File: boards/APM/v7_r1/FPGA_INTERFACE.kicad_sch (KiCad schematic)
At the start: 30 parts, among them J1 DF40C-60DS-0.4V(51), J15 FPGA FFC, J21 FPGA FMC, J3 DF40C-60DS-0.4V(51), J31 Conn_02x04_Odd_Even, SW1 RST

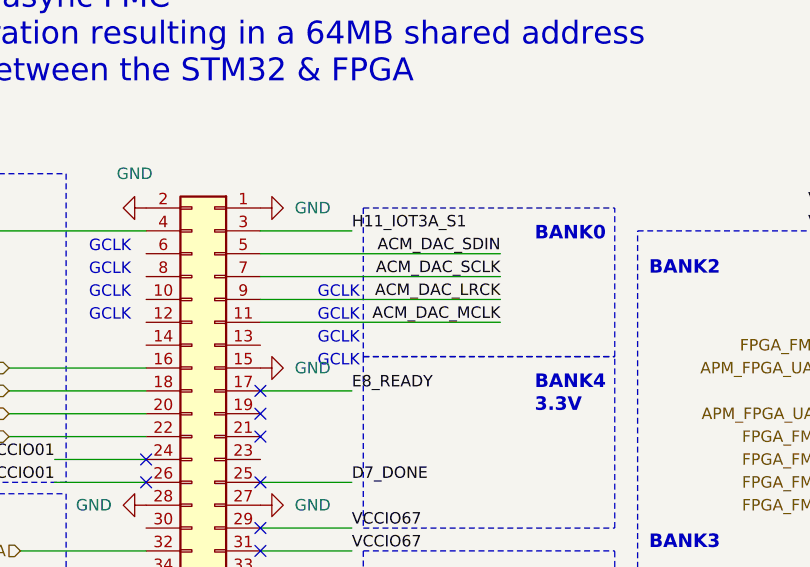
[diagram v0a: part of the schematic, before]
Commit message: floorplanning again
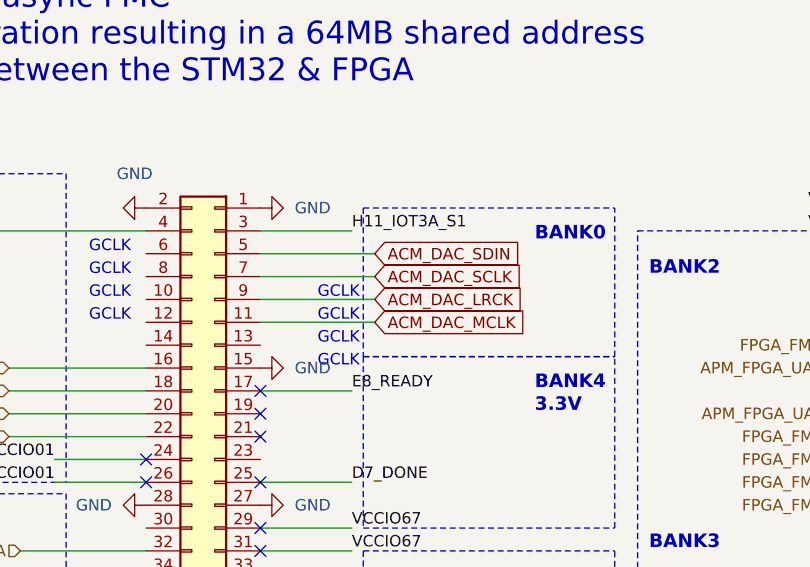
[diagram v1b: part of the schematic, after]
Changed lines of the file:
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@@
 	(wire
 		(pts
-			(xy 95.25 96.52) (xy 68.58 96.52)
+			(xy 81.28 96.52) (xy 68.58 96.52)
 		)
 		(stroke
@@
 	(wire
 		(pts
-			(xy 95.25 99.06) (xy 68.58 99.06)
+			(xy 81.28 99.06) (xy 68.58 99.06)
 		)
 		(stroke
@@
 	(wire
 		(pts
-			(xy 95.25 101.6) (xy 68.58 101.6)
+			(xy 81.28 101.6) (xy 68.58 101.6)
 		)
 		(stroke
@@
 	(wire
 		(pts
-			(xy 95.25 93.98) (xy 68.58 93.98)
+			(xy 81.28 93.98) (xy 68.58 93.98)
 		)
 		(stroke
@@
 		)
 	)
-	(label "ACM_DAC_MCLK"
-		(at 95.25 101.6 180)
-		(effects
-			(font
-				(size 1.27 1.27)
-			)
-			(justify right bottom)
-		)
-	)
 	(label "A3_JTAG_TDI"
 		(at 166.37 121.92 0)
@@
 		)
 	)
-	(label "ACM_DAC_LRCK"
-		(at 95.25 99.06 180)
-		(effects
-			(font
-				(size 1.27 1.27)
-			)
-			(justify right bottom)
-		)
-	)
 	(label "FPGA_3V3"
 		(at 137.16 149.86 180)
@@
 		)
 	)
-	(label "ACM_DAC_SDIN"
-		(at 95.25 93.98 180)
-		(effects
-			(font
-				(size 1.27 1.27)
-			)
-			(justify right bottom)
-		)
-	)
 	(label "FPGA_3V3"
 		(at 95.25 181.61 0)
@@
 		)
 	)
-	(label "ACM_DAC_SCLK"
-		(at 95.25 96.52 180)
-		(effects
-			(font
-				(size 1.27 1.27)
-			)
-			(justify right bottom)
-		)
-	)
 	(label "FPGA_3V3"
 		(at 137.16 147.32 180)
@@
 		)
 	)
+	(global_label "ACM_DAC_SCLK"
+		(shape input)
+		(at 81.28 96.52 0)
+		(fields_autoplaced yes)
+		(effects
+			(font
+				(size 1.27 1.27)
+			)
+			(justify left)
+		)
+		(property "Intersheetrefs" "${INTERSHEET_REFS}"
+			(at 98.4166 96.52 0)
+			(hide yes)
+			(show_name no)
+			(do_not_autoplace no)
+			(effects
+				(font
+					(size 1.27 1.27)
+				)
+				(justify left)
+			)
+		)
+	)
+	(global_label "ACM_DAC_SDIN"
+		(shape input)
+		(at 81.28 93.98 0)
+		(fields_autoplaced yes)
+		(effects
+			(font
+				(size 1.27 1.27)
+			)
+			(justify left)
+		)
+		(property "Intersheetrefs" "${INTERSHEET_REFS}"
+			(at 98.0538 93.98 0)
+			(hide yes)
+			(show_name no)
+			(do_not_autoplace no)
+			(effects
+				(font
+					(size 1.27 1.27)
+				)
+				(justify left)
+			)
+		)
+	)
+	(global_label "ACM_DAC_LRCK"
+		(shape input)
+		(at 81.28 99.06 0)
+		(fields_autoplaced yes)
+		(effects
+			(font
+				(size 1.27 1.27)
+			)
+			(justify left)
+		)
+		(property "Intersheetrefs" "${INTERSHEET_REFS}"
+			(at 98.4771 99.06 0)
+			(hide yes)
+			(show_name no)
+			(do_not_autoplace no)
+			(effects
+				(font
+					(size 1.27 1.27)
+				)
+				(justify left)
+			)
+		)
+	)
+	(global_label "ACM_DAC_MCLK"
+		(shape input)
+		(at 81.28 101.6 0)
+		(fields_autoplaced yes)
+		(effects
+			(font
+				(size 1.27 1.27)
+			)
+			(justify left)
+		)
+		(property "Intersheetrefs" "${INTERSHEET_REFS}"
+			(at 98.6585 101.6 0)
+			(hide yes)
+			(show_name no)
+			(do_not_autoplace no)
+			(effects
+				(font
+					(size 1.27 1.27)
+				)
+				(justify left)
+			)
+		)
+	)

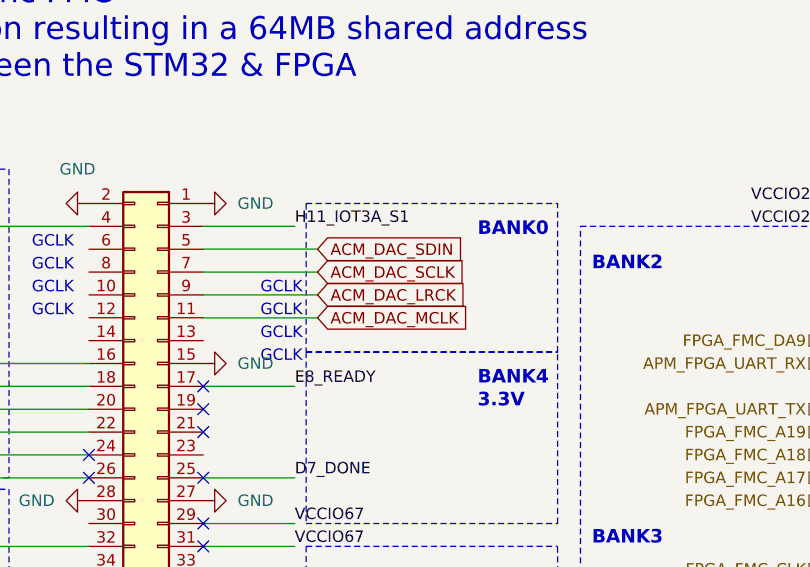
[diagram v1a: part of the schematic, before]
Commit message: more placement. starting fmc routing next
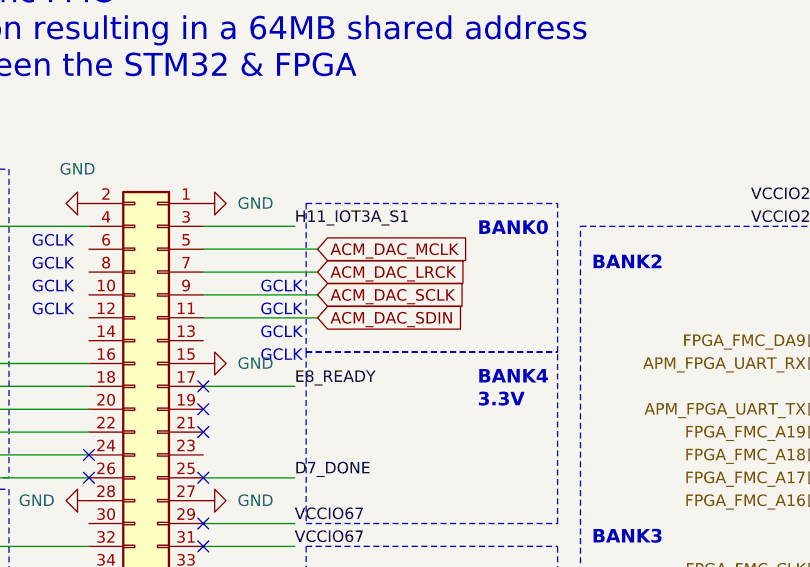
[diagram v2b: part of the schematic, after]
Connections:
- net ACM_DAC_LRCK: now also J1.7 (Pin_7); no longer J1.9 (Pin_9)
- net ACM_DAC_MCLK: now also J1.5 (Pin_5); no longer J1.11 (Pin_11)
- net ACM_DAC_SCLK: now also J1.9 (Pin_9); no longer J1.7 (Pin_7)
- net ACM_DAC_SDIN: now also J1.11 (Pin_11); no longer J1.5 (Pin_5)
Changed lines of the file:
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@@
 		)
 	)
-	(global_label "ACM_DAC_SCLK"
+	(global_label "ACM_DAC_MCLK"
 		(shape input)
-		(at 81.28 96.52 0)
+		(at 81.28 93.98 0)
 		(fields_autoplaced yes)
 		(effects
@@
 		)
 		(property "Intersheetrefs" "${INTERSHEET_REFS}"
-			(at 98.4166 96.52 0)
+			(at 98.6585 93.98 0)
 			(hide yes)
 			(show_name no)
@@
 	(global_label "ACM_DAC_SDIN"
 		(shape input)
-		(at 81.28 93.98 0)
+		(at 81.28 101.6 0)
 		(fields_autoplaced yes)
 		(effects
@@
 		)
 		(property "Intersheetrefs" "${INTERSHEET_REFS}"
-			(at 98.0538 93.98 0)
+			(at 98.0538 101.6 0)
+			(hide yes)
+			(show_name no)
+			(do_not_autoplace no)
+			(effects
+				(font
+					(size 1.27 1.27)
+				)
+				(justify left)
+			)
+		)
+	)
+	(global_label "ACM_DAC_SCLK"
+		(shape input)
+		(at 81.28 99.06 0)
+		(fields_autoplaced yes)
+		(effects
+			(font
+				(size 1.27 1.27)
+			)
+			(justify left)
+		)
+		(property "Intersheetrefs" "${INTERSHEET_REFS}"
+			(at 98.4166 99.06 0)
 			(hide yes)
 			(show_name no)
@@
 	(global_label "ACM_DAC_LRCK"
 		(shape input)
-		(at 81.28 99.06 0)
+		(at 81.28 96.52 0)
 		(fields_autoplaced yes)
 		(effects
@@
 		)
 		(property "Intersheetrefs" "${INTERSHEET_REFS}"
-			(at 98.4771 99.06 0)
+			(at 98.4771 96.52 0)
 			(hide yes)
 			(show_name no)
-			(do_not_autoplace no)
-			(effects
-				(font
-					(size 1.27 1.27)
-				)
-				(justify left)
-			)
-		)
-	)
-	(global_label "ACM_DAC_MCLK"
-		(shape input)
-		(at 81.28 101.6 0)
-		(fields_autoplaced yes)
-		(effects
-			(font
-				(size 1.27 1.27)
-			)
-			(justify left)
-		)
-		(property "Intersheetrefs" "${INTERSHEET_REFS}"
-			(at 98.6585 101.6 0)
-			(hide yes)
-			(show_name no)
